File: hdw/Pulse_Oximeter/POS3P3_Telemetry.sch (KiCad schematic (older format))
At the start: 11 parts, among them U501 INA219BxDCN, U502 MCP9804, U503 INA219BxDCN

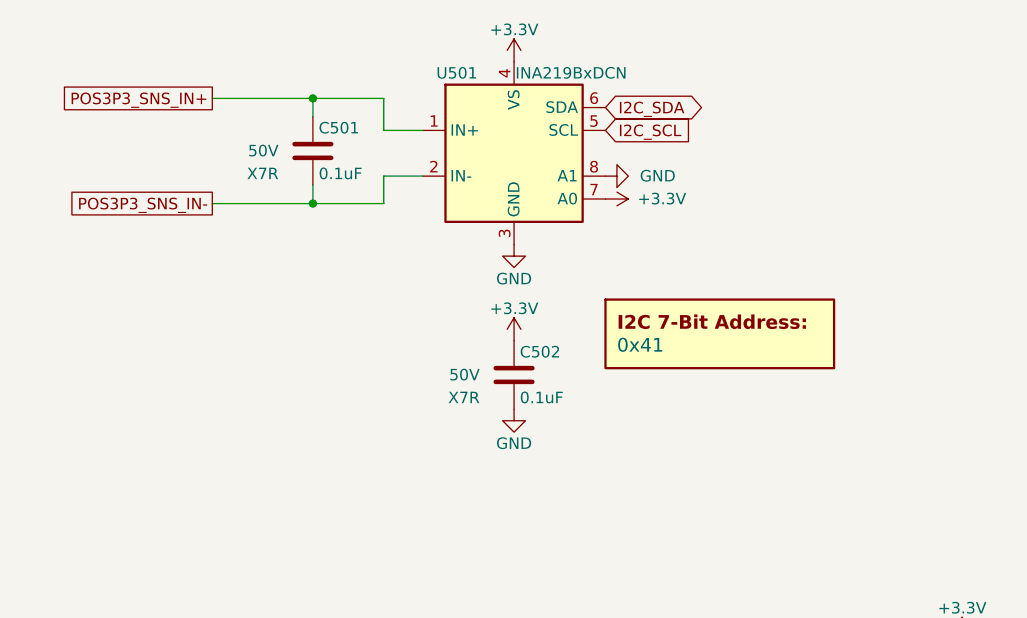
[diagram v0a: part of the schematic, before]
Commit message: More part arrangements
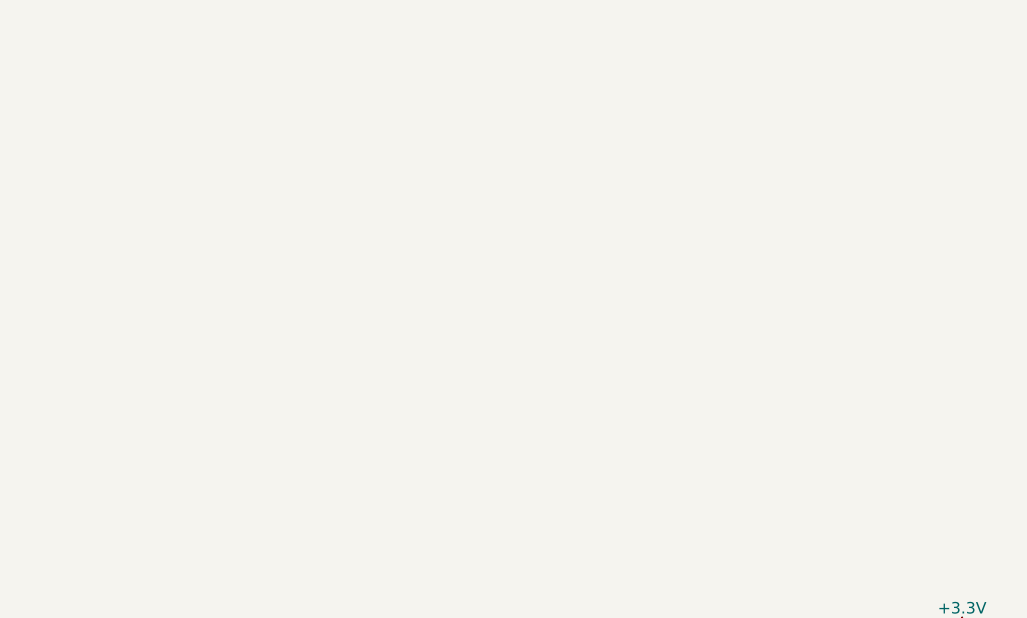
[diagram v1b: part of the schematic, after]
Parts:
- removed C501, C502: 0.1uF, Capacitors_SMD:C_0402, symbol Custom_Library:C_Custom
- removed DOC501: 0x41, symbol Custom_Library:I2C_Address
- removed U501: INA219BxDCN, Package_TO_SOT_SMD:SOT-23-8, symbol Analog_ADC:INA219BxDCN
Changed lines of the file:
@@
 $Descr A 11000 8500
 encoding utf-8
-Sheet 5 23
+Sheet 5 21
 Title "Pulse Oximeter"
 Date "2019-01-03"
@@
 Comment4 ""
 $EndDescr
-Text GLabel 2150 1970 0    50   UnSpc ~ 0
-POS3P3_SNS_IN+
-Text GLabel 2150 2430 0    50   UnSpc ~ 0
-POS3P3_SNS_IN-
 $Comp
 L power:GND #PWR?
@@
 $Comp
 L power:GND #PWR?
-U 1 1 5E1BD4BE
-P 3470 2610
-AR Path="/5E0652BA/5E1BD4BE" Ref="#PWR?"  Part="1"
-AR Path="/5E0A0E29/5E1BD4BE" Ref="#PWR?"  Part="1"
-AR Path="/5E052856/5E1BD4BE" Ref="#PWR?"  Part="1"
-AR Path="/5EAE2DDC/5E1BD4BE" Ref="#PWR0502"  Part="1"
-F 0 "#PWR0502" H 3470 2360 50  0001 C CNN
-F 1 "GND" H 3470 2460 50  0000 C CNN
-F 2 "" H 3470 2610 50  0001 C CNN
-F 3 "" H 3470 2610 50  0001 C CNN
-	1    3470 2610
-	1    0    0    -1
-$EndComp
-$Comp
-L power:+3.3V #PWR?
-U 1 1 5EC52D0E
-P 3470 1810
-AR Path="/5E0652BA/5EC52D0E" Ref="#PWR?"  Part="1"
-AR Path="/5E0A0E29/5EC52D0E" Ref="#PWR?"  Part="1"
-AR Path="/5E052856/5EC52D0E" Ref="#PWR?"  Part="1"
-AR Path="/5EAE2DDC/5EC52D0E" Ref="#PWR0501"  Part="1"
-F 0 "#PWR0501" H 3470 1660 50  0001 C CNN
-F 1 "+3.3V" H 3470 1950 50  0000 C CNN
-F 2 "" H 3470 1810 50  0001 C CNN
-F 3 "" H 3470 1810 50  0001 C CNN
-	1    3470 1810
-	1    0    0    -1
-$EndComp
-Text GLabel 3870 2110 2    50   Input ~ 0
-I2C_SCL
-$Comp
-L Custom_Library:C_Custom C?
-U 1 1 5EC52D0F
-P 3470 3180
-AR Path="/5B3E071A/5EC52D0F" Ref="C?"  Part="1"
-AR Path="/5E0652BA/5EC52D0F" Ref="C?"  Part="1"
-AR Path="/5E0A0E29/5EC52D0F" Ref="C?"  Part="1"
-AR Path="/5E052856/5EC52D0F" Ref="C?"  Part="1"
-AR Path="/5EAE2DDC/5EC52D0F" Ref="C502"  Part="1"
-F 0 "C502" H 3495 3280 50  0000 L CNN
-F 1 "0.1uF" H 3495 3080 50  0000 L CNN
-F 2 "Capacitors_SMD:C_0402" H 3508 3030 50  0001 C CNN
-F 3 "" H 3495 3280 50  0001 C CNN
-F 4 "" H 3320 3280 50  0000 R CNN "display_footprint"
-F 5 "50V" H 3320 3180 50  0000 R CNN "Voltage"
-F 6 "X7R" H 3320 3080 50  0000 R CNN "Dielectric"
-F 7 "490-10701-1-ND" H -440 -3700 50  0001 C CNN "Digi-Key PN"
-	1    3470 3180
-	1    0    0    -1
-$EndComp
-$Comp
-L power:+3.3V #PWR?
-U 1 1 5EC52D10
-P 3470 3030
-AR Path="/5E0652BA/5EC52D10" Ref="#PWR?"  Part="1"
-AR Path="/5E0A0E29/5EC52D10" Ref="#PWR?"  Part="1"
-AR Path="/5E052856/5EC52D10" Ref="#PWR?"  Part="1"
-AR Path="/5EAE2DDC/5EC52D10" Ref="#PWR0503"  Part="1"
-F 0 "#PWR0503" H 3470 2880 50  0001 C CNN
-F 1 "+3.3V" H 3470 3170 50  0000 C CNN
-F 2 "" H 3470 3030 50  0001 C CNN
-F 3 "" H 3470 3030 50  0001 C CNN
-	1    3470 3030
-	1    0    0    -1
-$EndComp
-$Comp
-L power:GND #PWR?
-U 1 1 5EC52D11
-P 3470 3330
-AR Path="/5E0652BA/5EC52D11" Ref="#PWR?"  Part="1"
-AR Path="/5E0A0E29/5EC52D11" Ref="#PWR?"  Part="1"
-AR Path="/5E052856/5EC52D11" Ref="#PWR?"  Part="1"
-AR Path="/5EAE2DDC/5EC52D11" Ref="#PWR0504"  Part="1"
-F 0 "#PWR0504" H 3470 3080 50  0001 C CNN
-F 1 "GND" H 3470 3180 50  0000 C CNN
-F 2 "" H 3470 3330 50  0001 C CNN
-F 3 "" H 3470 3330 50  0001 C CNN
-	1    3470 3330
-	1    0    0    -1
-$EndComp
-Text GLabel 3870 2010 2    50   BiDi ~ 0
-I2C_SDA
-$Comp
-L Custom_Library:I2C_Address DOC?
-U 1 1 5E1BD4E2
-P 4370 3050
-AR Path="/5E0652BA/5E1BD4E2" Ref="DOC?"  Part="1"
-AR Path="/5E0A0E29/5E1BD4E2" Ref="DOC?"  Part="1"
-AR Path="/5E052856/5E1BD4E2" Ref="DOC?"  Part="1"
-AR Path="/5EAE2DDC/5E1BD4E2" Ref="DOC501"  Part="1"
-F 0 "DOC501" H 4370 3300 60  0001 C CNN
-F 1 "0x41" H 3920 3050 60  0000 L CNN
-F 2 "" H 4370 3400 60  0001 C CNN
-F 3 "" H 4370 3400 60  0001 C CNN
-	1    4370 3050
-	1    0    0    -1
-$EndComp
-Wire Wire Line
-	2590 2430 2590 2350
-Wire Wire Line
-	2590 2050 2590 1970
-$Comp
-L Custom_Library:C_Custom C?
-U 1 1 5EC52D12
-P 2590 2200
-AR Path="/5B3E071A/5EC52D12" Ref="C?"  Part="1"
-AR Path="/5E0652BA/5EC52D12" Ref="C?"  Part="1"
-AR Path="/5E0A0E29/5EC52D12" Ref="C?"  Part="1"
-AR Path="/5E052856/5EC52D12" Ref="C?"  Part="1"
-AR Path="/5EAE2DDC/5EC52D12" Ref="C501"  Part="1"
-F 0 "C501" H 2615 2300 50  0000 L CNN
-F 1 "0.1uF" H 2615 2100 50  0000 L CNN
-F 2 "Capacitors_SMD:C_0402" H 2628 2050 50  0001 C CNN
-F 3 "" H 2615 2300 50  0001 C CNN
-F 4 "" H 2440 2300 50  0000 R CNN "display_footprint"
-F 5 "50V" H 2440 2200 50  0000 R CNN "Voltage"
-F 6 "X7R" H 2440 2100 50  0000 R CNN "Dielectric"
-F 7 "490-10701-1-ND" H -1320 -4680 50  0001 C CNN "Digi-Key PN"
-	1    2590 2200
-	1    0    0    -1
-$EndComp
-Wire Wire Line
-	2150 2430 2590 2430
-Wire Wire Line
-	2150 1970 2590 1970
-Wire Wire Line
-	3070 2110 2900 2110
-Wire Wire Line
-	2900 2110 2900 1970
-Wire Wire Line
-	2900 1970 2590 1970
-Connection ~ 2590 1970
-Wire Wire Line
-	3070 2310 2900 2310
-Wire Wire Line
-	2900 2310 2900 2430
-Wire Wire Line
-	2900 2430 2590 2430
-Connection ~ 2590 2430
-$Comp
-L power:GND #PWR?
 U 1 1 5EC52D14
 P 8180 2610
@@
 Connection ~ 7300 2430
 $Comp
-L Analog_ADC:INA219BxDCN U501
-U 1 1 5EC52D13
-P 3470 2210
-F 0 "U501" H 3220 2560 50  0000 C CNN
-F 1 "INA219BxDCN" H 3720 2560 50  0000 C CNN
-F 2 "Package_TO_SOT_SMD:SOT-23-8" H 4120 1860 50  0001 C CNN
-F 3 "http://www.ti.com/lit/ds/symlink/ina219.pdf" H 3820 2110 50  0001 C CNN
-F 4 "296-46420-1-ND" H 3470 2210 50  0001 C CNN "Digi-Key PN"
-F 5 "Telemetry" H 3470 2210 50  0001 C CNN "Configuration"
-	1    3470 2210
-	1    0    0    -1
-$EndComp
-$Comp
-L power:GND #PWR0505
-U 1 1 5E32642A
-P 3870 2310
-F 0 "#PWR0505" H 3870 2060 50  0001 C CNN
-F 1 "GND" V 3870 2160 50  0000 R CNN
-F 2 "" H 3870 2310 50  0001 C CNN
-F 3 "" H 3870 2310 50  0001 C CNN
-	1    3870 2310
-	0    -1   -1   0
-$EndComp
-$Comp
-L power:+3.3V #PWR0506
-U 1 1 5E326B95
-P 3870 2410
-F 0 "#PWR0506" H 3870 2260 50  0001 C CNN
-F 1 "+3.3V" V 3870 2550 50  0000 L CNN
-F 2 "" H 3870 2410 50  0001 C CNN
-F 3 "" H 3870 2410 50  0001 C CNN
-	1    3870 2410
-	0    1    1    0
-$EndComp
-$Comp
 L power:GND #PWR0518
